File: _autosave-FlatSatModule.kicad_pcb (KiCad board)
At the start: 4 copper layers, 110.2 x 119.4 mm, 8 parts, among them J1 DB26_Male_HighDensity_Mountin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, J2 Micro_SD_Card_Det, J3 HEADER_13x2

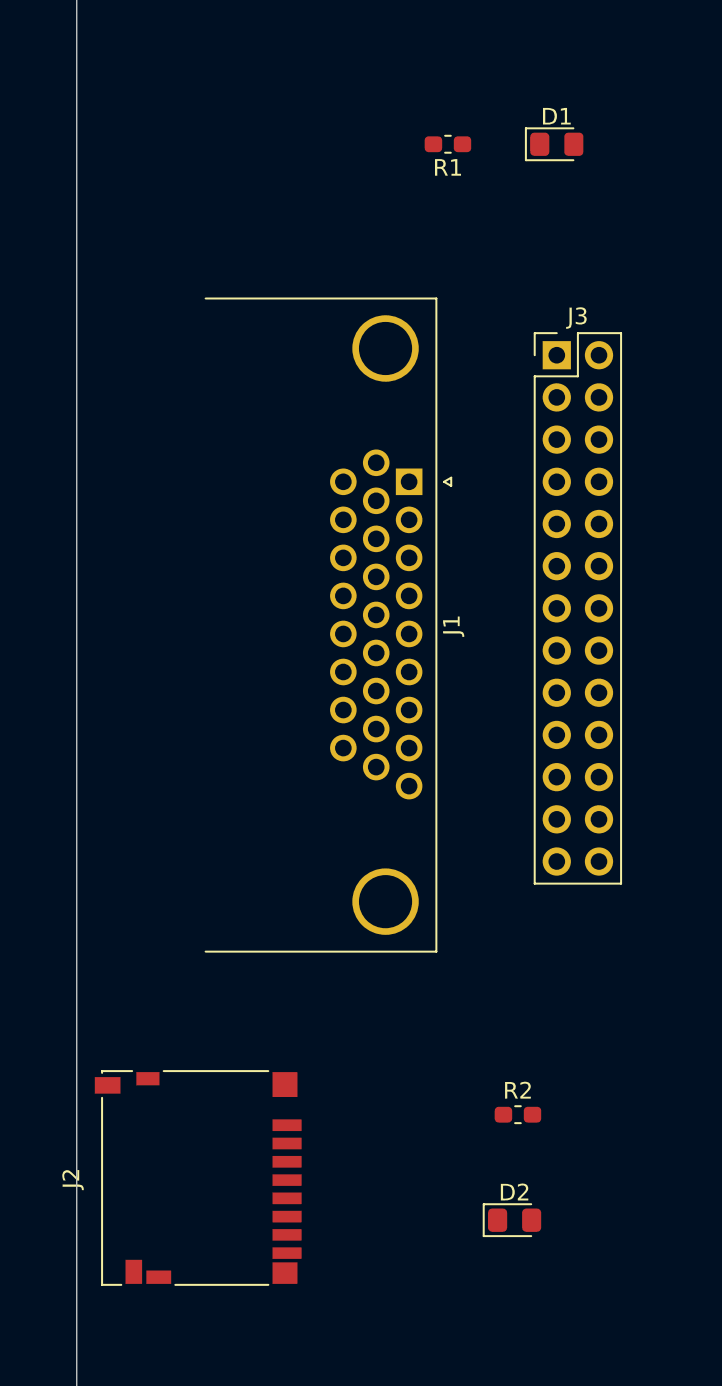
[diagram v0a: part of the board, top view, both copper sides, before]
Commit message: clarify schematic
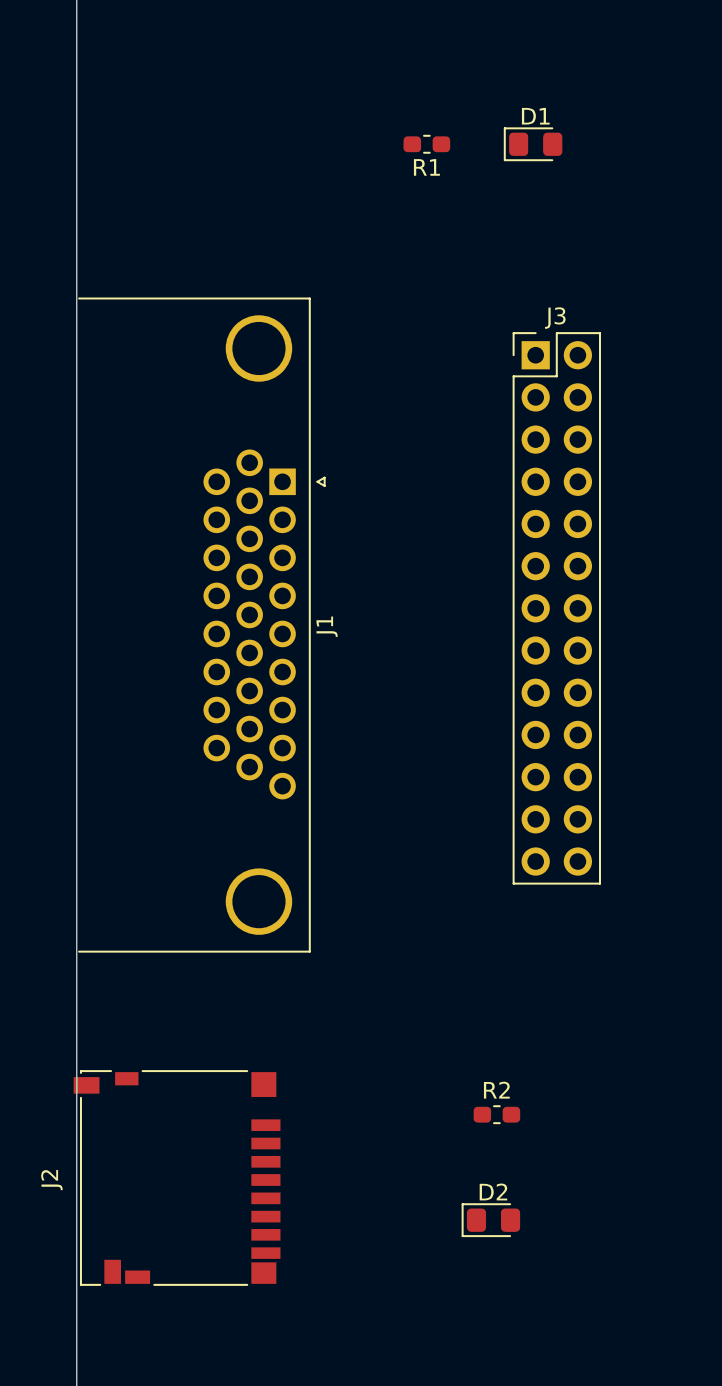
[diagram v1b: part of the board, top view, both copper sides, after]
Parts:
- moved J1 7.62 mm to (72.4, 76.2)
- moved D1 1.27 mm to (87.6, 55.9)
- moved J3 1.27 mm to (87.6, 68.6)
- moved D2 1.27 mm to (85.1, 120.7)
- moved J2 1.27 mm to (66.0, 118.1)
- moved R1 1.27 mm to (81.1, 55.9)
- moved R2 1.27 mm to (85.3, 114.3)
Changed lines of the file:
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@@
   )
   (module Connector_PinHeader_2.54mm:PinHeader_2x13_P2.54mm_Vertical (layer F.Cu)
-    (at 88.9 68.58)
+    (at 87.63 68.58)
     (descr "Through hole straight pin header, 2x13, 2.54mm pitch, double rows")
     (tags "Through hole pin header THT 2x13 2.54mm double row")
@@
   )
   (module Connector_Dsub:DSUB-26-HD_Male_Horizontal_P2.29x1.98mm_EdgePinOffset8.35mm_Housed_MountingHolesOffset10.89mm (layer F.Cu)
-    (at 80.01 76.2 270)
+    (at 72.39 76.2 270)
     (descr "26-pin D-Sub connector, horizontal/angled (90 deg), THT-mount, male, pitch 2.29x1.98mm, pin-PCB-offset 8.35mm, distance of mounting holes 33.3mm, distance of mounting holes to PCB edge 10.889999999999999mm, see https://disti-assets.s3.amazonaws.com/tonar/files/datasheets/16730.pdf")
     (tags "26-pin D-Sub connector horizontal angled 90deg THT male pitch 2.29x1.98mm pin-PCB-offset 8.35mm mounting-holes-distance 33.3mm mounting-hole-offset 33.3mm")
@@
   )
   (module Resistor_SMD:R_0603_1608Metric_Pad1.05x0.95mm_HandSolder (layer F.Cu)
-    (at 86.5625 114.3)
+    (at 85.2925 114.3)
     (descr "Resistor SMD 0603 (1608 Metric), square (rectangular) end terminal, IPC_7351 nominal with elongated pad for handsoldering. (Body size source: http://www.tortai-tech.com/upload/download/2011102023233369053.pdf), generated with kicad-footprint-generator")
     (tags "resistor handsolder")
@@
   )
   (module Resistor_SMD:R_0603_1608Metric_Pad1.05x0.95mm_HandSolder (layer F.Cu)
-    (at 82.3475 55.88 180)
+    (at 81.0775 55.88 180)
     (descr "Resistor SMD 0603 (1608 Metric), square (rectangular) end terminal, IPC_7351 nominal with elongated pad for handsoldering. (Body size source: http://www.tortai-tech.com/upload/download/2011102023233369053.pdf), generated with kicad-footprint-generator")
     (tags "resistor handsolder")
@@
   )
   (module LED_SMD:LED_0805_2012Metric_Pad1.15x1.40mm_HandSolder (layer F.Cu)
-    (at 86.36 120.65)
+    (at 85.09 120.65)
     (descr "LED SMD 0805 (2012 Metric), square (rectangular) end terminal, IPC_7351 nominal, (Body size source: https://docs.google.com/spreadsheets/d/1BsfQQcO9C6DZCsRaXUlFlo91Tg2WpOkGARC1WS5S8t0/edit?usp=sharing), generated with kicad-footprint-generator")
     (tags "LED handsolder")
@@
   )
   (module LED_SMD:LED_0805_2012Metric_Pad1.15x1.40mm_HandSolder (layer F.Cu)
-    (at 88.9 55.88)
+    (at 87.63 55.88)
     (descr "LED SMD 0805 (2012 Metric), square (rectangular) end terminal, IPC_7351 nominal, (Body size source: https://docs.google.com/spreadsheets/d/1BsfQQcO9C6DZCsRaXUlFlo91Tg2WpOkGARC1WS5S8t0/edit?usp=sharing), generated with kicad-footprint-generator")
     (tags "LED handsolder")
@@
   )
   (module Connector_Card:microSD_HC_Hirose_DM3D-SF (layer F.Cu)
-    (at 67.31 118.11 90)
+    (at 66.04 118.11 90)
     (descr "Micro SD, SMD, right-angle, push-pull (https://media.digikey.com/PDF/Data%20Sheets/Hirose%20PDFs/DM3D-SF.pdf)")
     (tags "Micro SD")
